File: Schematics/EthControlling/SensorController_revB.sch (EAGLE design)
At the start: 31 parts, among them IC2 MEGA164P/324P/644P-AU, IC4 4066D, Q1 20.000M

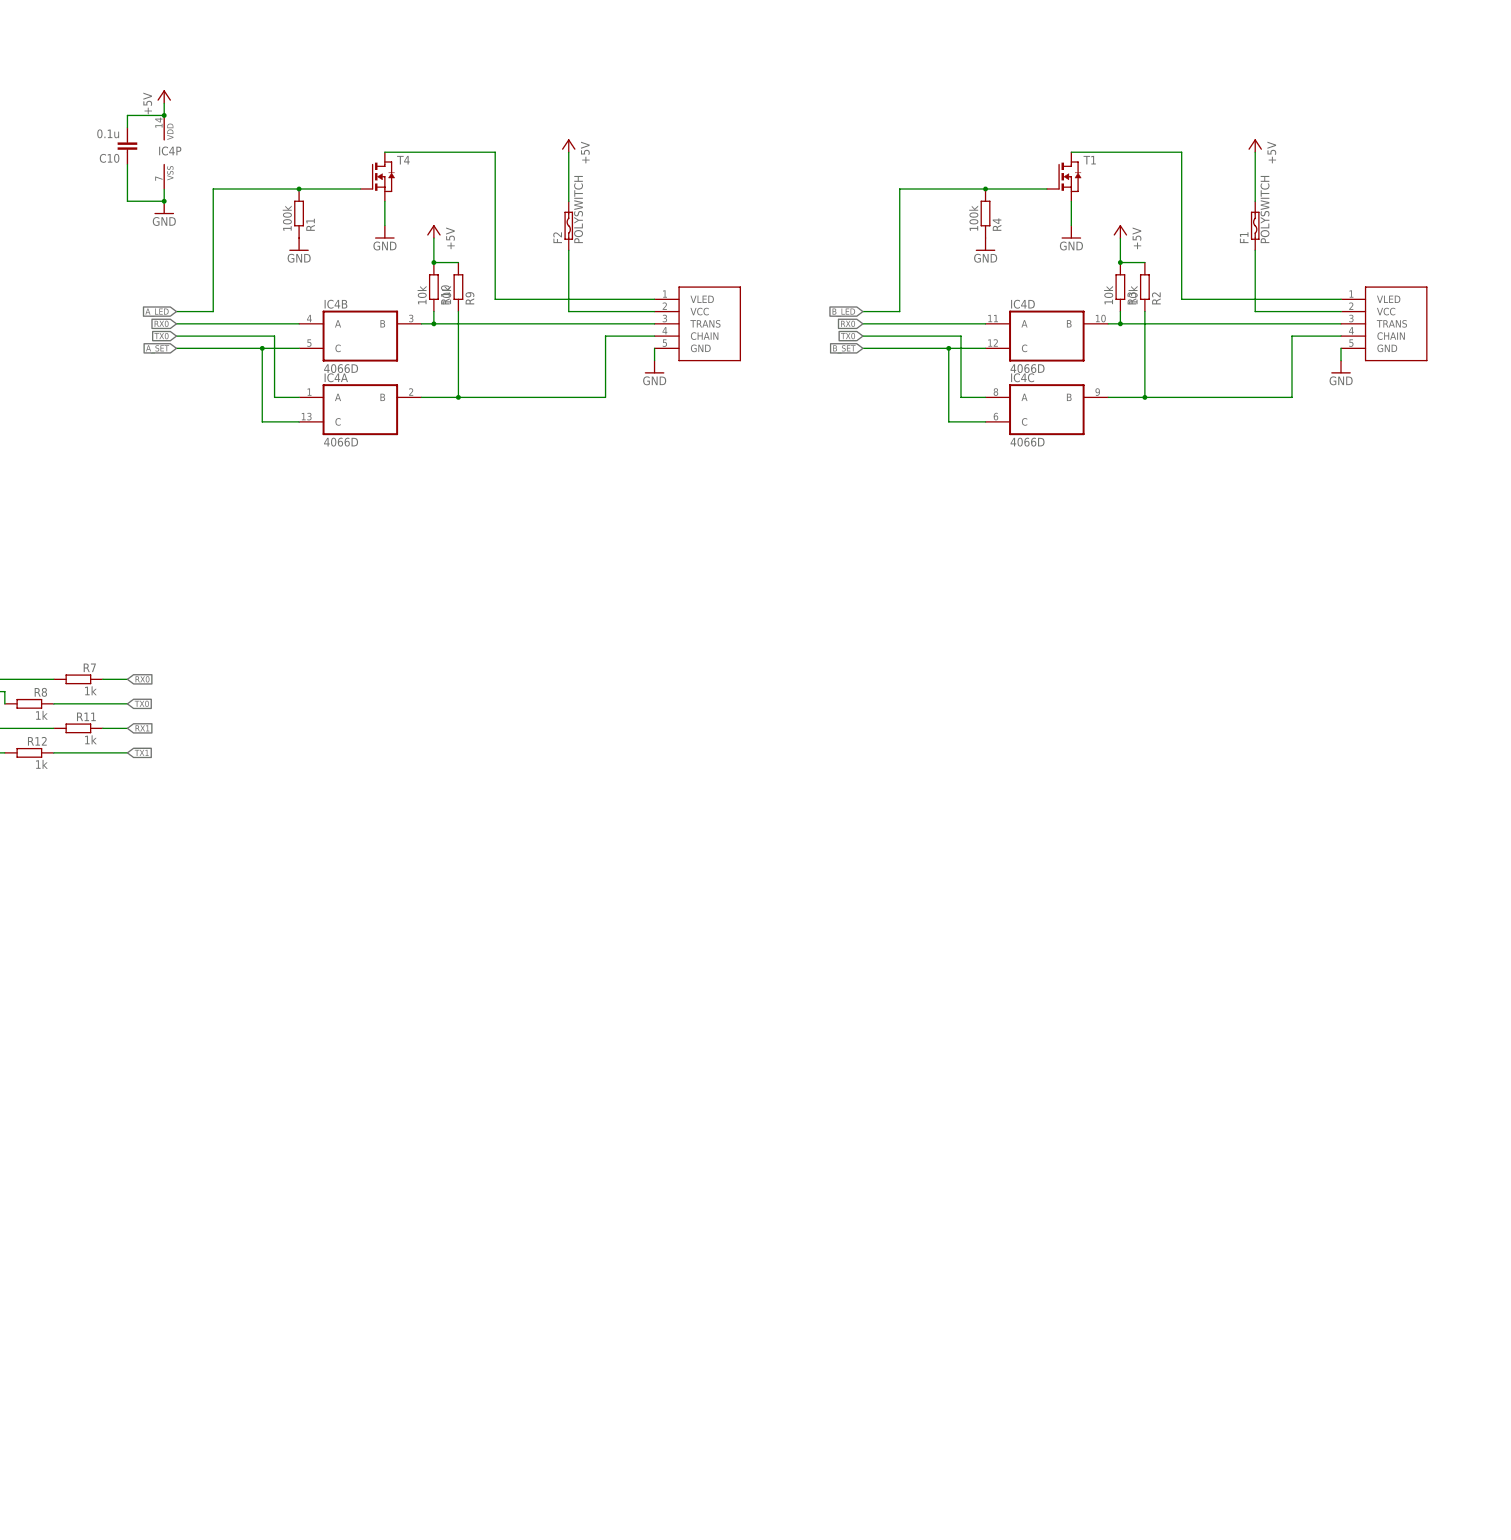
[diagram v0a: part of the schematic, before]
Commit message: ditto
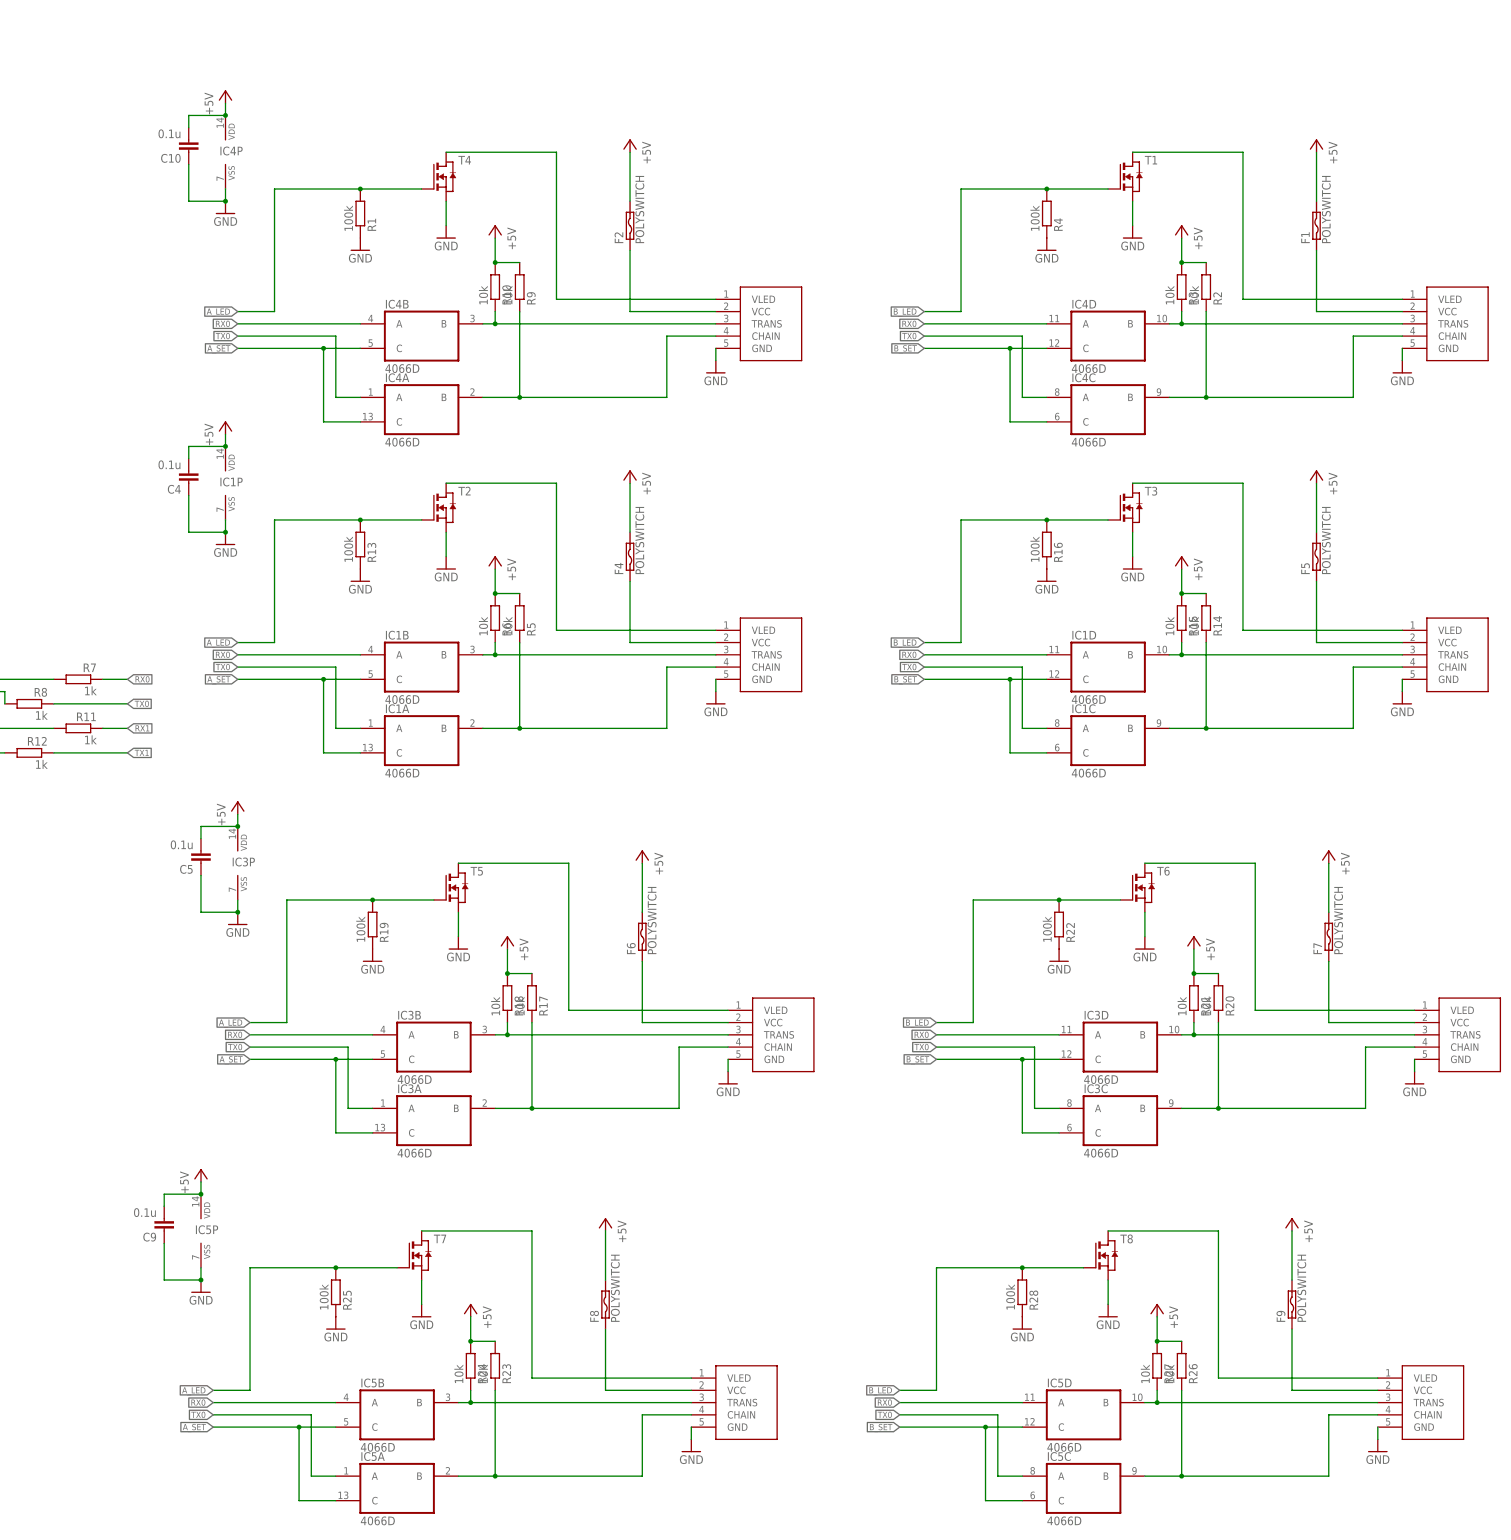
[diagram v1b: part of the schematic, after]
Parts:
- added A_OUT1, A_OUT2, A_OUT3, B_OUT1, B_OUT2, B_OUT3: SERIAL_SENSORXH, myparts:SERIAL_SENSORXH
- added C4, C5, C9: 0.1u, rcl:C-EUC1608
- added F4, F5, F6, F7, F8, F9: POLYSWITCH, myparts:POLYSWITCH
- added IC1, IC3, IC5: 4066D, 40xx:4066D
- added R13, R16, R19, R22, R25, R28: 100k, rcl:R-EU_R0603
- added R14, R15, R17, R18, R20, R21, R23, R24, R26, R27, R5, R6: 10k, rcl:R-EU_R0603
- added T2, T3, T5, T6, T7, T8: (no value), zetex:NMOSSOT23
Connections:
- new net N$11: A_OUT1.TRANS, IC1B.B, R6.1
- new net N$12: A_OUT1.VCC, F4.1
- new net N$13: A_OUT1.VLED, T2.D
- new net N$14: B_OUT1.CHAIN, IC1C.B, R14.1
- new net N$15: B_OUT1.TRANS, IC1D.B, R15.1
- new net N$16: B_OUT1.VCC, F5.1
- new net N$19: B_OUT1.VLED, T3.D
- new net N$24: A_OUT2.CHAIN, IC3A.B, R17.1
- new net N$25: A_OUT2.TRANS, IC3B.B, R18.1
- new net N$26: A_OUT2.VCC, F6.1
- new net N$27: A_OUT2.VLED, T5.D
- new net N$28: B_OUT2.CHAIN, IC3C.B, R20.1
- new net N$29: B_OUT2.TRANS, IC3D.B, R21.1
- new net N$30: B_OUT2.VCC, F7.1
- new net N$31: B_OUT2.VLED, T6.D
- new net N$32: A_OUT3.CHAIN, IC5A.B, R23.1
- new net N$33: A_OUT3.TRANS, IC5B.B, R24.1
- new net N$34: A_OUT3.VCC, F8.1
- new net N$35: A_OUT3.VLED, T7.D
- new net N$36: B_OUT3.CHAIN, IC5C.B, R26.1
- new net N$37: B_OUT3.TRANS, IC5D.B, R27.1
- new net N$38: B_OUT3.VCC, F9.1
- new net N$39: B_OUT3.VLED, T8.D
- new net N$8: A_OUT1.CHAIN, IC1A.B, R5.1
- net +5V: now also C4.2, C5.2, C9.2, F4.2, F5.2, F6.2, F7.2, F8.2, F9.2, IC1P.VDD, IC3P.VDD, IC5P.VDD, R14.2, R15.2, R17.2, R18.2, R20.2, R21.2, R23.2, R24.2, R26.2, R27.2, R5.2, R6.2
- net A_LED: now also R13.2, R19.2, R25.2, T2.G, T5.G, T7.G
- net A_SET: now also IC1A.C, IC1B.C, IC3A.C, IC3B.C, IC5A.C, IC5B.C
- net B_LED: now also R16.2, R22.2, R28.2, T3.G, T6.G, T8.G
- net B_SET: now also IC1C.C, IC1D.C, IC3C.C, IC3D.C, IC5C.C, IC5D.C
- net GND: now also A_OUT1.GND, A_OUT2.GND, A_OUT3.GND, B_OUT1.GND, B_OUT2.GND, B_OUT3.GND, C4.1, C5.1, C9.1, IC1P.VSS, IC3P.VSS, IC5P.VSS, R13.1, R16.1, R19.1, R22.1, R25.1, R28.1, T2.S, T3.S, T5.S, T6.S, T7.S, T8.S
- net RX0: now also IC1B.A, IC1D.A, IC3B.A, IC3D.A, IC5B.A, IC5D.A
- net TX0: now also IC1A.A, IC1C.A, IC3A.A, IC3C.A, IC5A.A, IC5C.A
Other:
- moved on the sheet: C10, F1, F2, IC4A, IC4B, IC4C, IC4D, IC4P, R1, R10, R2, R3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
